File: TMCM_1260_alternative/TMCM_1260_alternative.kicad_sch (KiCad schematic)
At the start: 111 parts, among them J1 Motor, J2 CAN, J3 I/O, J4 Power, J5 USB_B_Micro, J7 Conn_01x05, Q1 NVMFD5C650NLT1G, Q2 NVMFD5C650NLT1G, Q3 NVMFD5C650NLT1G, Q4 NVMFD5C650NLT1G, U1 LMZM23600V3SILR, U2 STM32F091CCTx, U3 TCAN337, U4 TMC5160A-TA-T, U5 AS5047P-ATSM, U6 24LC02, U7 CP2102N-Axx-xQFN24, Y1 Crystal_Small

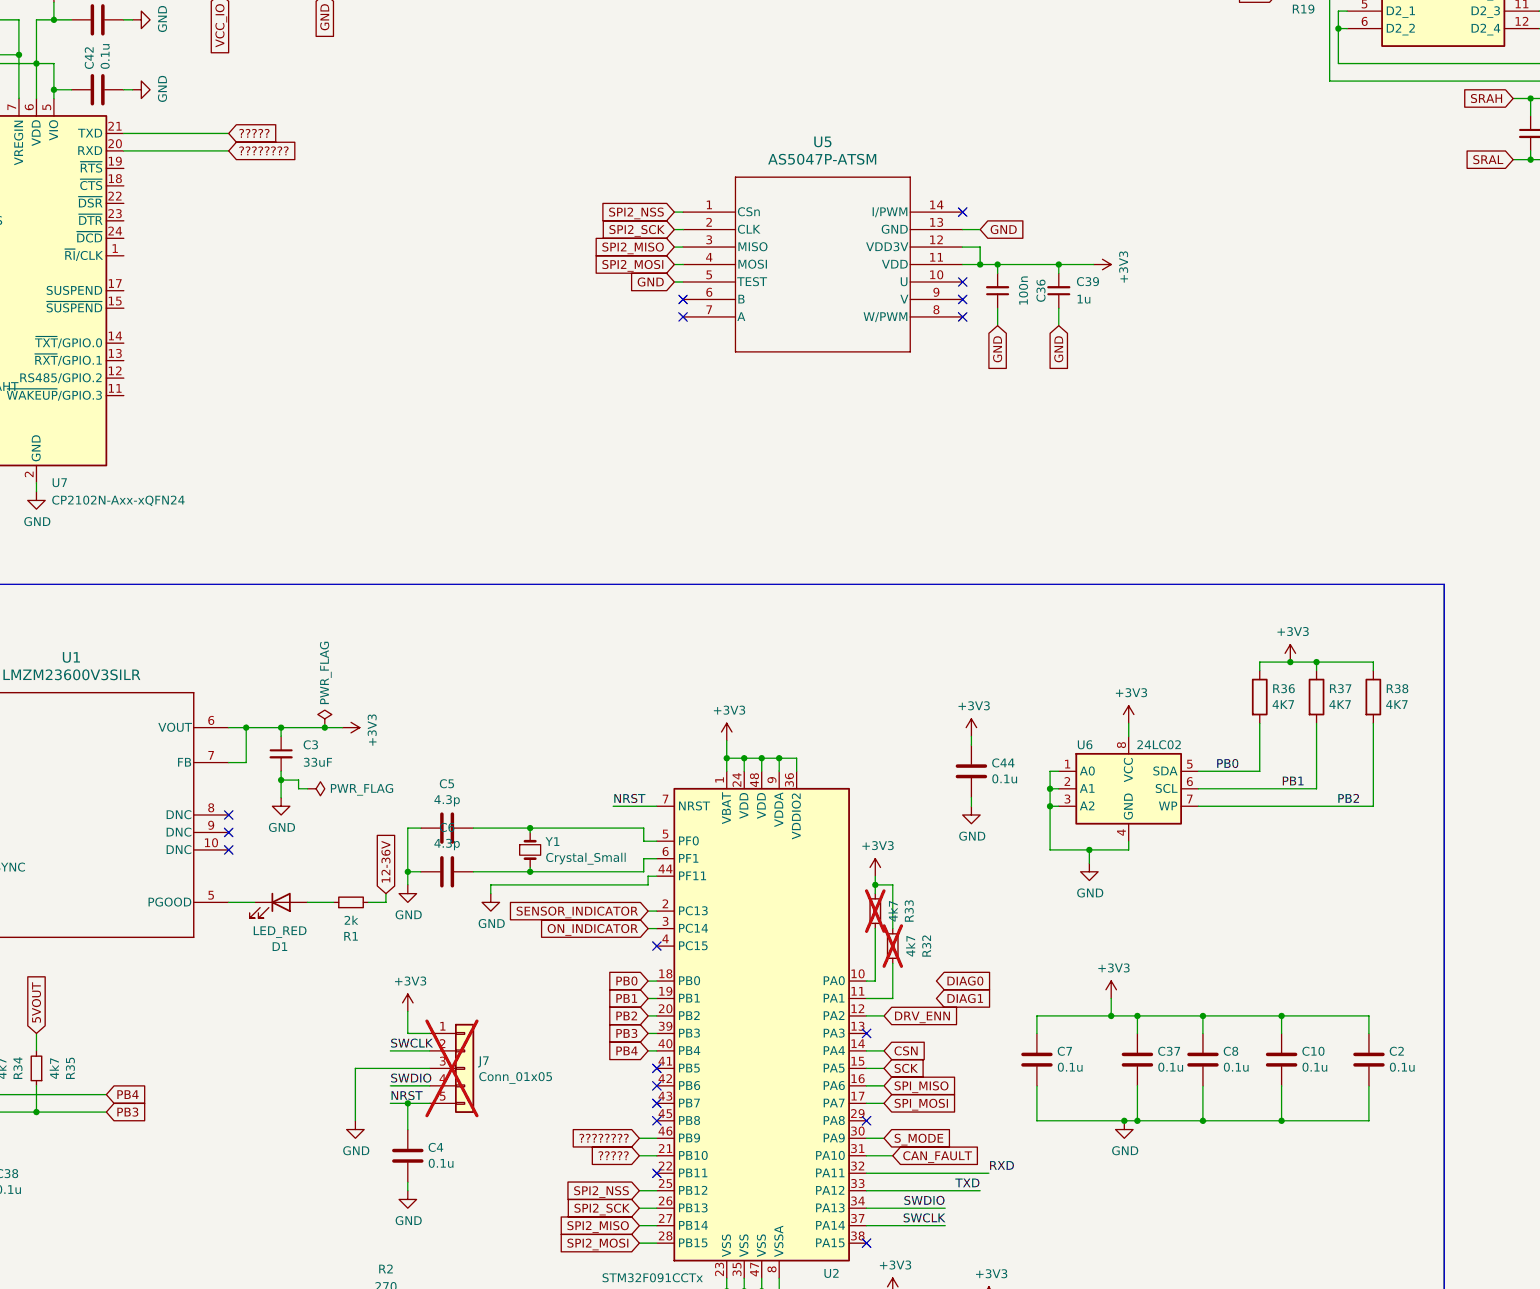
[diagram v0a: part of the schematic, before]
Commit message: finished
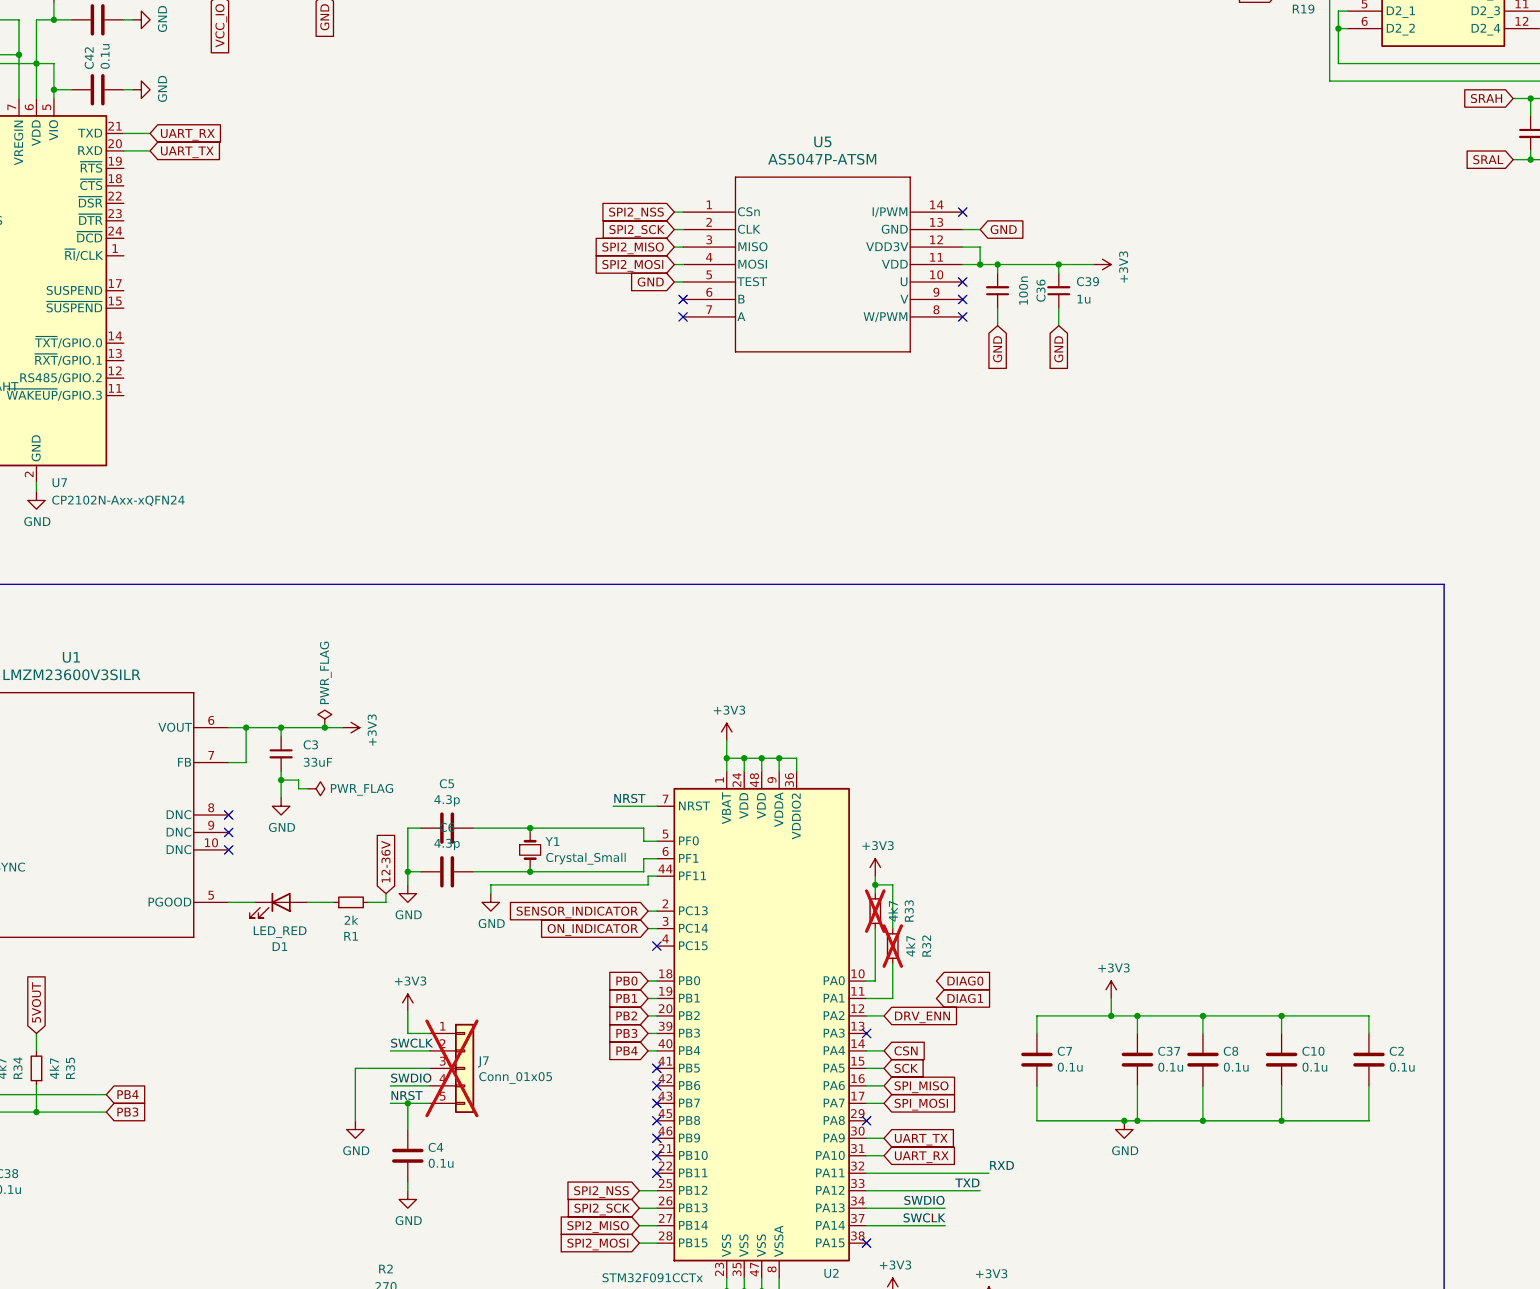
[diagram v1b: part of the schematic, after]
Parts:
- removed C44: 0.1u, Capacitor_SMD:C_0603_1608Metric_Pad1.08x0.95mm_HandSolder, symbol Device:C
- removed R36, R37, R38: 4K7, Resistor_SMD:R_0603_1608Metric, symbol Device:R
- removed U6: 24LC02, Housings_SOIC:SOIC-8_3.9x4.9mm_Pitch1.27mm, symbol Memory_EEPROM:24LC02
- U7: PN (none) -> CP2102N-A02-GQFN24R
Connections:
- net CAN_FAULT: no longer U2.31 (PA10)
- net ?????: no longer names the net of U2.21 (PB10)
- net ?????: no longer U7.21 (TXD)
- net ????????: no longer names the net of U2.46 (PB9)
- net ????????: no longer U7.20 (RXD)
- net S_MODE renamed UART_TX
- net UART_TX: now also U7.20 (RXD)
- new net UART_RX: U2.31 (PA10), U7.21 (TXD)
- no-connect marks 26 -> 28
